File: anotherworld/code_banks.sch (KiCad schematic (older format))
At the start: 3 parts

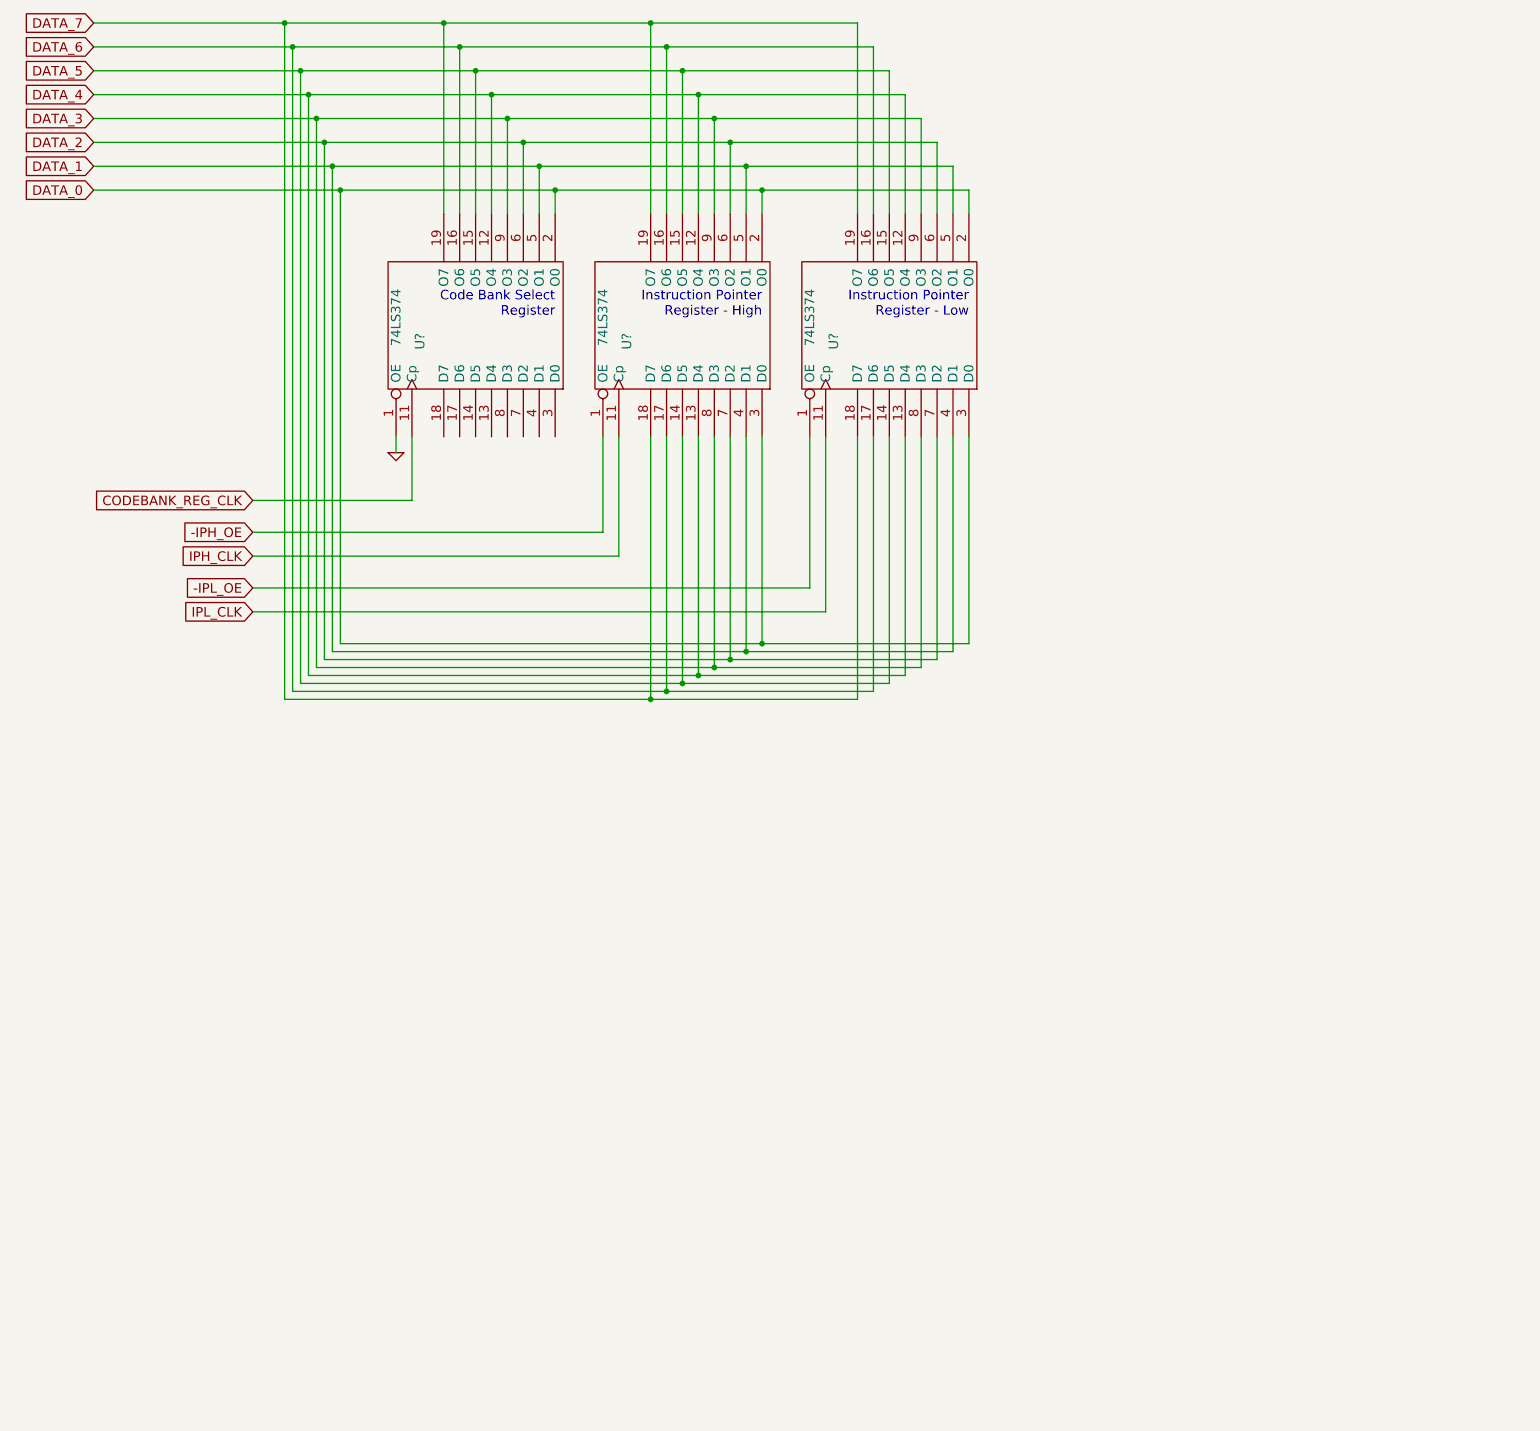
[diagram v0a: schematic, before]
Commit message: lots of stuff :-)
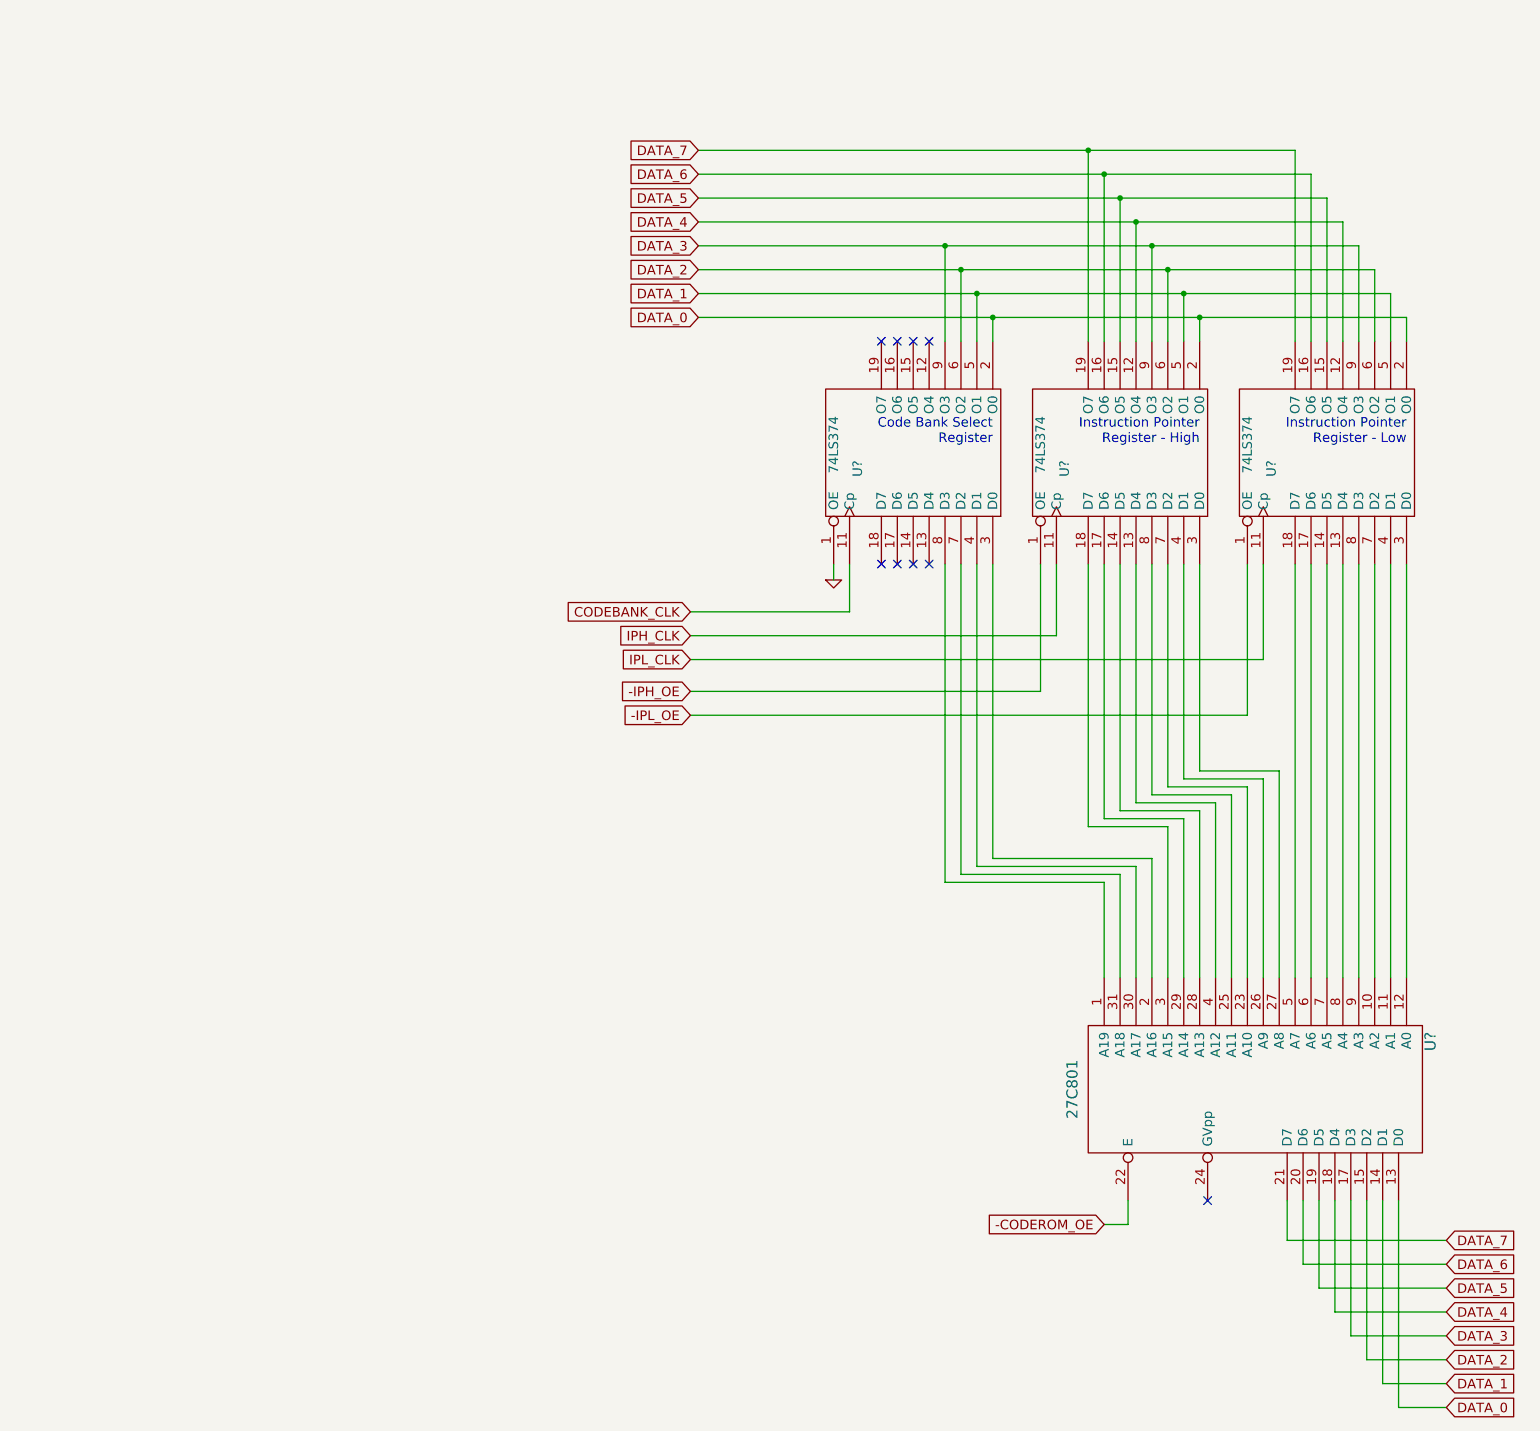
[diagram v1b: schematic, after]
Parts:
- added U?: 27C801, ~, symbol 27C801
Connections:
- net DATA_0: now also U?.13 (D0); no longer U?.3 (D0), U?.3 (D0)
- net DATA_1: now also U?.14 (D1); no longer U?.4 (D1), U?.4 (D1)
- net DATA_2: now also U?.15 (D2); no longer U?.7 (D2), U?.7 (D2)
- net DATA_3: now also U?.17 (D3); no longer U?.8 (D3), U?.8 (D3)
- net DATA_4: now also U?.18 (D4); no longer U?.12 (O4), U?.13 (D4), U?.13 (D4)
- net DATA_5: now also U?.19 (D5); no longer U?.14 (D5), U?.14 (D5), U?.15 (O5)
- net DATA_6: now also U?.20 (D6); no longer U?.16 (O6), U?.17 (D6), U?.17 (D6)
- net DATA_7: now also U?.21 (D7); no longer U?.18 (D7), U?.18 (D7), U?.19 (O7)
- net GND: now also U?.16 (GND)
- net VCC: now also U?.32 (VCC)
- net at U?.3 (D0): now also U?.2 (A16)
- net at U?.4 (D1): now also U?.30 (A17)
- net at U?.7 (D2): now also U?.31 (A18)
- net at U?.8 (D3): now also U?.1 (A19)
- net CODEBANK_REG_CLK renamed CODEBANK_CLK
- new net: U?.10 (A2), U?.7 (D2)
- new net: U?.11 (A1), U?.4 (D1)
- new net: U?.12 (A0), U?.3 (D0)
- new net: U?.23 (A10), U?.7 (D2)
- new net: U?.25 (A11), U?.8 (D3)
- new net: U?.26 (A9), U?.4 (D1)
- new net: U?.27 (A8), U?.3 (D0)
- new net: U?.14 (D5), U?.28 (A13)
- new net: U?.17 (D6), U?.29 (A14)
- new net: U?.18 (D7), U?.3 (A15)
- new net: U?.13 (D4), U?.4 (A12)
- new net: U?.18 (D7), U?.5 (A7)
- new net: U?.17 (D6), U?.6 (A6)
- new net: U?.14 (D5), U?.7 (A5)
- new net: U?.13 (D4), U?.8 (A4)
- new net: U?.8 (D3), U?.9 (A3)
- new net -CODEROM_OE: U?.22 (E)
- no-connect marks 0 -> 9
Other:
- moved on the sheet: U?
